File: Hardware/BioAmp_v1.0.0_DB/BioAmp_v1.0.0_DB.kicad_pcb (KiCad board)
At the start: 2 copper layers, 120 x 33 mm, 23 parts, among them CN1 CKCL44X7R1H, CN2 CKCL44X7R1H, CN3 CKCL44X7R1H, J10 Jack_Touch-Proof, J2 Jack_Touch-Proof, J3 Jack_Touch-Proof, J4 Jack_Touch-Proof, J5 Jack_Touch-Proof, J6 Jack_Touch-Proof, J7 Jack_Touch-Proof, J8 Jack_Touch-Proof, J9 Jack_Touch-Proof, P1 CONN_01X10, U1 TPD4E1B06, U2 TPD4E1B06, U3 TPD4E1B06

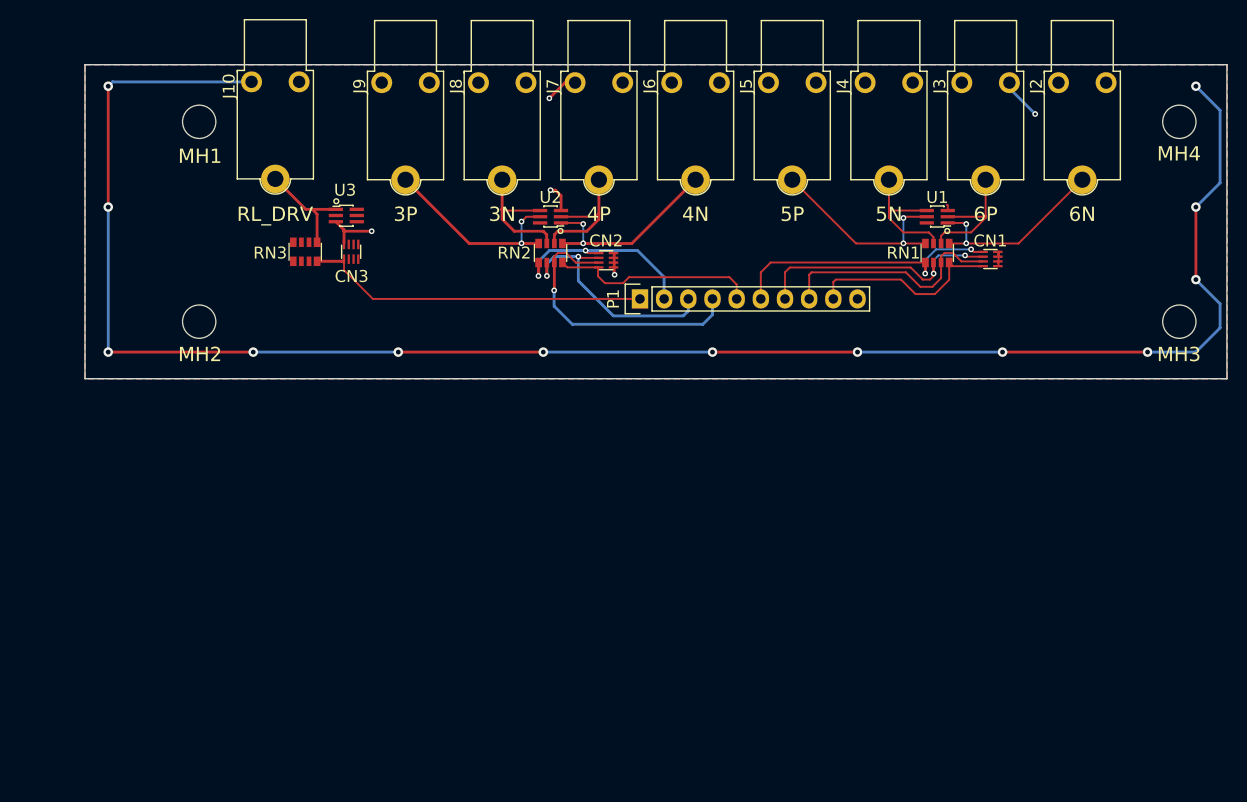
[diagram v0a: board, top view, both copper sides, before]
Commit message: Update Hardware/Bioamp_v1.0.0_DB: Project Folder Tree
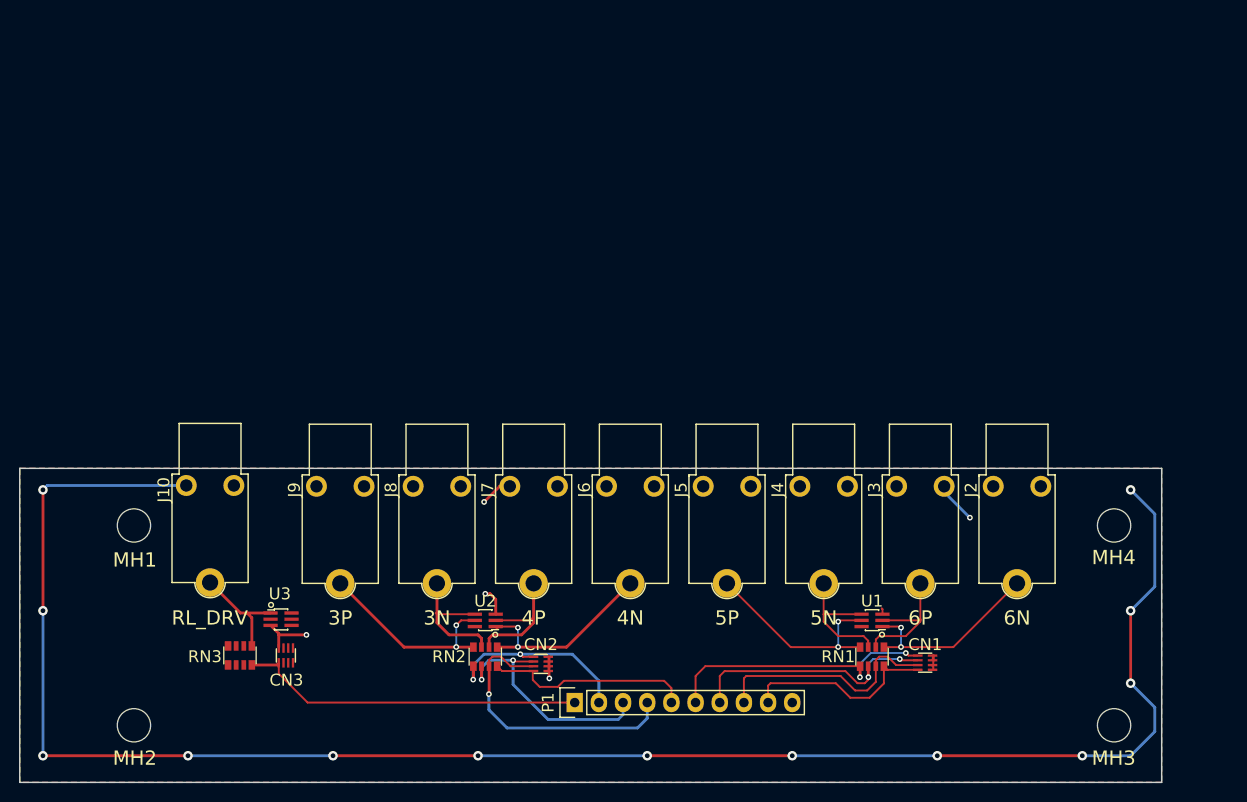
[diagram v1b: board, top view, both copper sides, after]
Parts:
- moved J10 43.0 mm to (102.1, 95.4)
- moved J2 43.0 mm to (186.9, 95.5)
- moved J3 43.0 mm to (176.8, 95.5)
- moved J4 43.0 mm to (166.6, 95.5)
- moved J5 43.0 mm to (156.5, 95.5)
- moved J6 43.0 mm to (146.3, 95.5)
- moved J7 43.0 mm to (136.1, 95.5)
- moved J8 43.0 mm to (126.0, 95.5)
- moved J9 43.0 mm to (115.8, 95.5)
- moved MH1 43.0 mm to (94.1, 94.4)
- moved MH2 43.0 mm to (94.1, 115.4)
- moved MH3 43.0 mm to (197.1, 115.4)
- moved MH4 43.0 mm to (197.1, 94.4)
- moved P1 43.0 mm to (140.5, 113.0)
- moved U1 43.0 mm to (171.7, 104.4)
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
